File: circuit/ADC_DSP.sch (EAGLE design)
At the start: 54 parts, among them IC1 REG1117, IC2 AD8605, IC3 STM32F40XRXT6, IC4 CS4272, Q1 8MHz, Q2 24.576MHz

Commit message: - ?????????? ??????
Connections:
- net N$16 renamed AINB+
- net N$17 renamed AINA+
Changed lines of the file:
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@@
 </segment>
 </net>
-<net name="N$16" class="0">
+<net name="AINB+" class="0">
 <segment>
 <pinref part="IC4" gate="G$1" pin="AINB+"/>
@@
 </segment>
 </net>
-<net name="N$17" class="0">
+<net name="AINA+" class="0">
 <segment>
 <pinref part="IC4" gate="G$1" pin="AINA+"/>

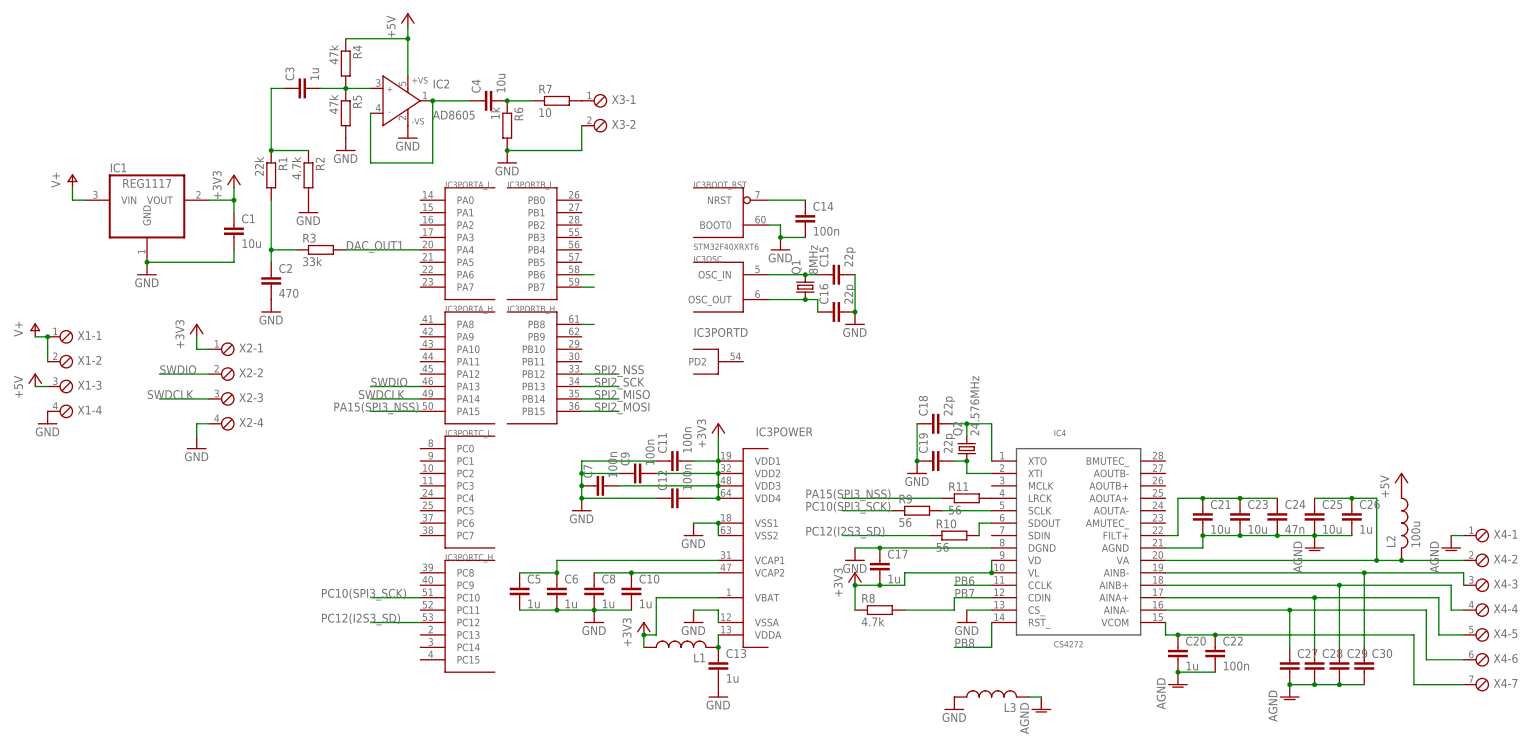
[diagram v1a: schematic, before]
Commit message: - ???????? ???????????? ADC_DSP.sch
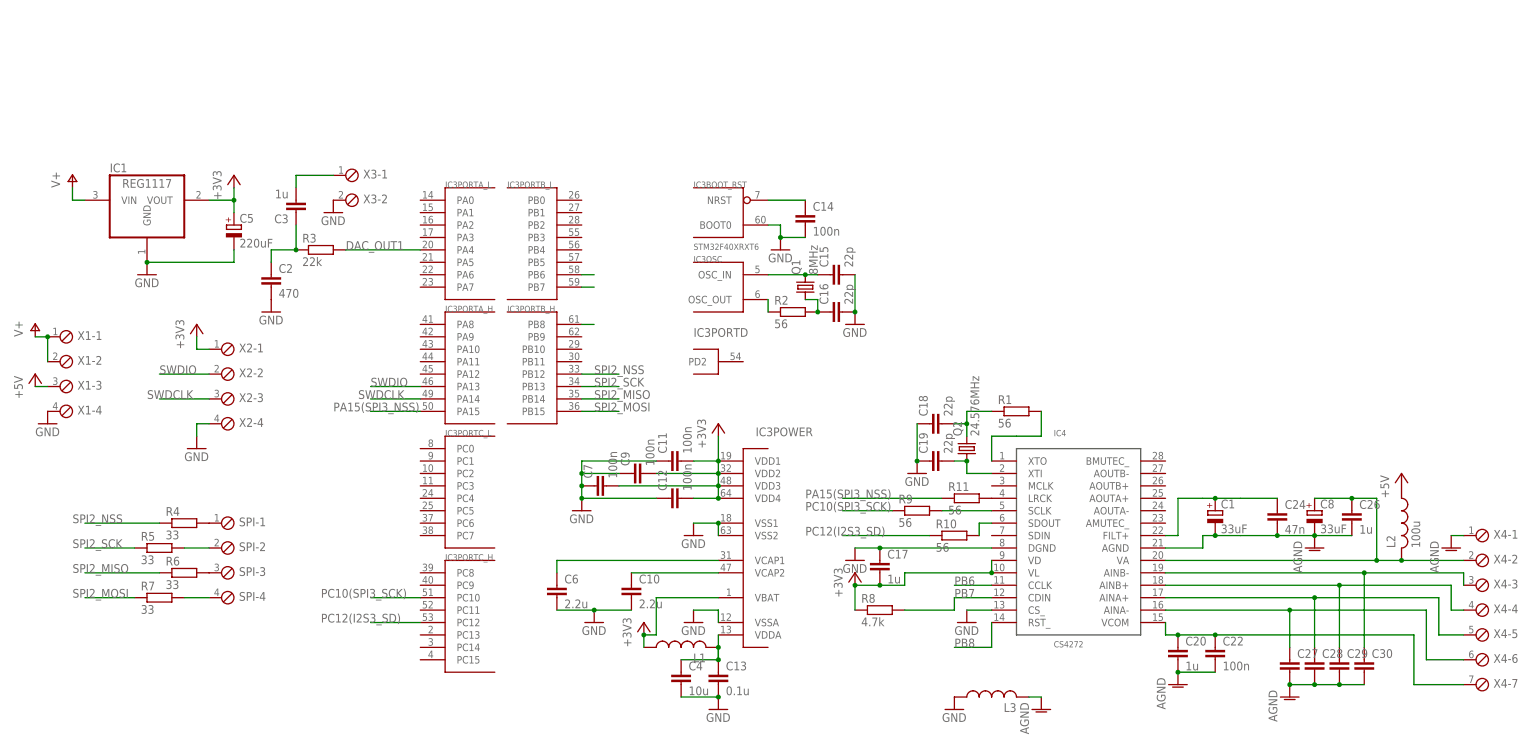
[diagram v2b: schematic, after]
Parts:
- removed C21, C23, C25: 10u, rcl:C-EUC0805
- removed IC2: AD8605, analog-devices:AD8603UJ
- added SPI: (no value), con-phoenix-254:MPT4
- C1: value 10u -> 33uF; device rcl:C-EUC0805 -> rcl:CPOL-EU153CLV-0605
- C10, C6: value 1u -> 2.2u
- C13: value 1u -> 0.1u
- C5: value 1u -> 220uF; device rcl:C-EUC0603 -> rcl:CPOL-EU153CLV-0605
- C8: value 1u -> 33uF; device rcl:C-EUC0603 -> rcl:CPOL-EU153CLV-0605
- R1: value 22k -> 56
- R2: value 4.7k -> 56
- R3: value 33k -> 22k
- R4, R5: value 47k -> 33
- R6: value 1k -> 33
- R7: value 10 -> 33
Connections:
- new net N$16: C3.2, X3-1.1
- new net N$17: IC4.XTO, R1.2
- net +3V3: now also C5.+; no longer C1.1
- net +5V: no longer IC2.+VS, R4.1
- net AGND: now also C1.-, C8.-; no longer C21.2, C23.2, C25.2
- net AVCC: now also C8.+; no longer C25.1
- net GND: now also C4.2, C5.-; no longer C1.2, C5.2, C8.2, IC2.-VS, R2.2, R5.2, R6.2
- net N$1: no longer C8.1
- net N$12: now also C1.+; no longer C21.1, C23.1
- net N$19: now also IC3OSC.OSC_OUT, R2.1; no longer C4.1, IC2.IN-, IC2.OUT
- net N$2: no longer C5.1
- net N$20: now also R4.2, SPI-1.1; no longer C4.2, R6.1, R7.1
- net N$21: now also R5.2, SPI-2.1; no longer R7.2, X3-1.1
- net N$22: now also R6.2, SPI-3.1; no longer C3.2, IC2.IN+, R4.2, R5.1
- net N$23: now also C3.1; no longer R1.2
- net N$24: now also R7.2, SPI-4.1; no longer C3.1, R1.1, R2.1
- net N$3: now also C4.1
- net N$6: now also R2.2; no longer IC3OSC.OSC_OUT
- net N$8: now also R1.1; no longer IC4.XTO
- net SPI2_MISO: now also R6.1
- net SPI2_MOSI: now also R7.1
- net SPI2_NSS: now also R4.1
- net SPI2_SCK: now also R5.1
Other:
- moved on the sheet: C13, C3, C4, R1, R2, R4, R5, R6, R7, X3-1, X3-2
